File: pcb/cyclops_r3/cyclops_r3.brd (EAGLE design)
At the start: 69.8 x 53.3 mm, 78 parts, among them Q1 SUM11006, Q2 IRF540, U1 MCP4921, U2 317-N, U3 TLV37, U4 337-N, U5 ADR03, U6 OP1177, U7 TLV2374, U8 ZXTD45

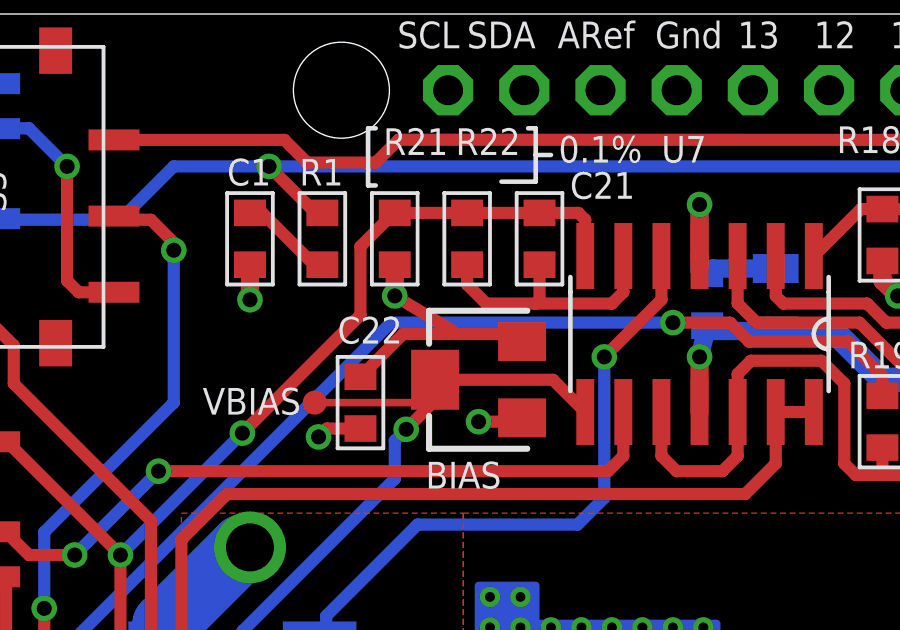
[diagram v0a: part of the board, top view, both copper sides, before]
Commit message: Minor fix to pcb.
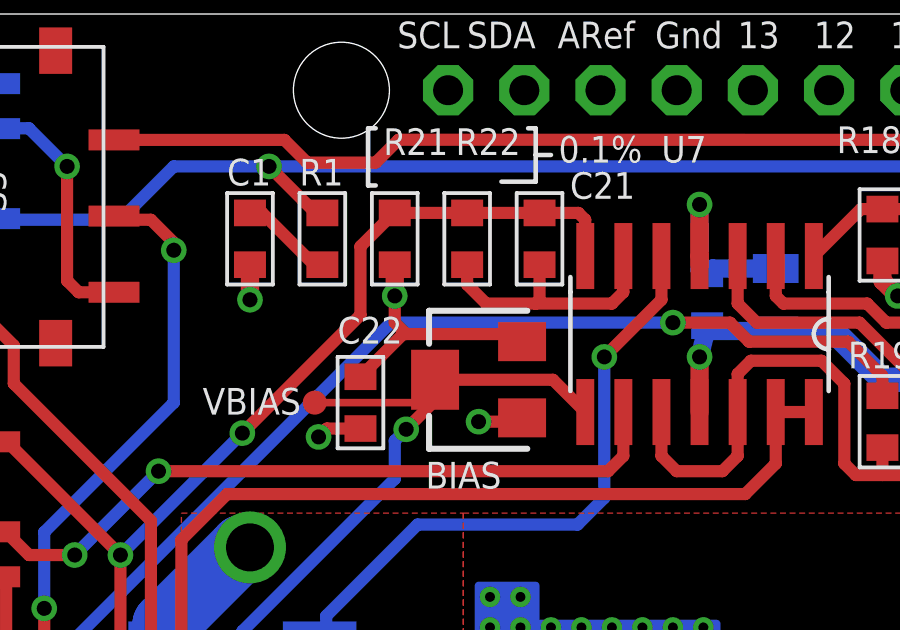
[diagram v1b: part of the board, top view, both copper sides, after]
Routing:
- net GND: track 102.9 -> 102.0 mm
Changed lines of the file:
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@@
 <layer number="27" name="tValues" color="7" fill="1" visible="yes" active="yes"/>
 <layer number="28" name="bValues" color="7" fill="1" visible="yes" active="yes"/>
-<layer number="29" name="tStop" color="7" fill="3" visible="no" active="yes"/>
-<layer number="30" name="bStop" color="7" fill="6" visible="no" active="yes"/>
+<layer number="29" name="tStop" color="7" fill="3" visible="yes" active="yes"/>
+<layer number="30" name="bStop" color="7" fill="6" visible="yes" active="yes"/>
 <layer number="31" name="tCream" color="7" fill="4" visible="no" active="yes"/>
 <layer number="32" name="bCream" color="7" fill="5" visible="no" active="yes"/>
@@
 <contactref element="C22" pad="2"/>
 <wire x1="15.875" y1="41.2496" x2="17.2974" y2="42.672" width="0.4064" layer="1"/>
-<wire x1="17.2974" y1="42.672" x2="18.796" y2="42.672" width="0.4064" layer="1"/>
-<wire x1="18.796" y1="42.672" x2="20.701" y2="42.672" width="0.4064" layer="1"/>
+<wire x1="17.2974" y1="42.672" x2="20.701" y2="42.672" width="0.4064" layer="1"/>
 <wire x1="20.701" y1="42.672" x2="20.955" y2="42.418" width="0.4064" layer="1"/>
 <wire x1="20.955" y1="42.418" x2="21.262" y2="42.418" width="0.4064" layer="1"/>
@@
 <wire x1="50.546" y1="37.719" x2="50.546" y2="39.37" width="0.8128" layer="1"/>
 <via x="40.64" y="43.688" extent="1-16" drill="0.9" shape="octagon"/>
-<wire x1="17.018" y1="43.942" x2="18.923" y2="42.799" width="0.4064" layer="1"/>
-<wire x1="18.923" y1="42.799" x2="18.796" y2="42.672" width="0.4064" layer="1" curve="-90"/>
+<wire x1="17.018" y1="43.942" x2="17.018" y2="43.053" width="0.4064" layer="1"/>
+<wire x1="17.018" y1="43.053" x2="17.399" y2="42.672" width="0.4064" layer="1"/>
 <wire x1="66.008" y1="11.459" x2="66.008" y2="11.144" width="0.4064" layer="1"/>
 <wire x1="58.547" y1="8.382" x2="58.166" y2="8.001" width="0.4064" layer="1"/>
@@
 <via x="38.989" y="30.226" extent="1-16" drill="0.9" shape="octagon"/>
 <wire x1="38.989" y1="28.575" x2="38.989" y2="30.226" width="0.8128" layer="1"/>
+<wire x1="17.399" y1="42.672" x2="17.2974" y2="42.672" width="0" layer="19" extent="1-1"/>
 </signal>
 <signal name="VIN">
@@
 </signal>
 </signals>
-<errors>
-</errors>
 </board>
 </drawing>
